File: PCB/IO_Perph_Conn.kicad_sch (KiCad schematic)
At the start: 18 parts, among them U301 STM32MP157FABx, Y601 NX2012SA-32.768K

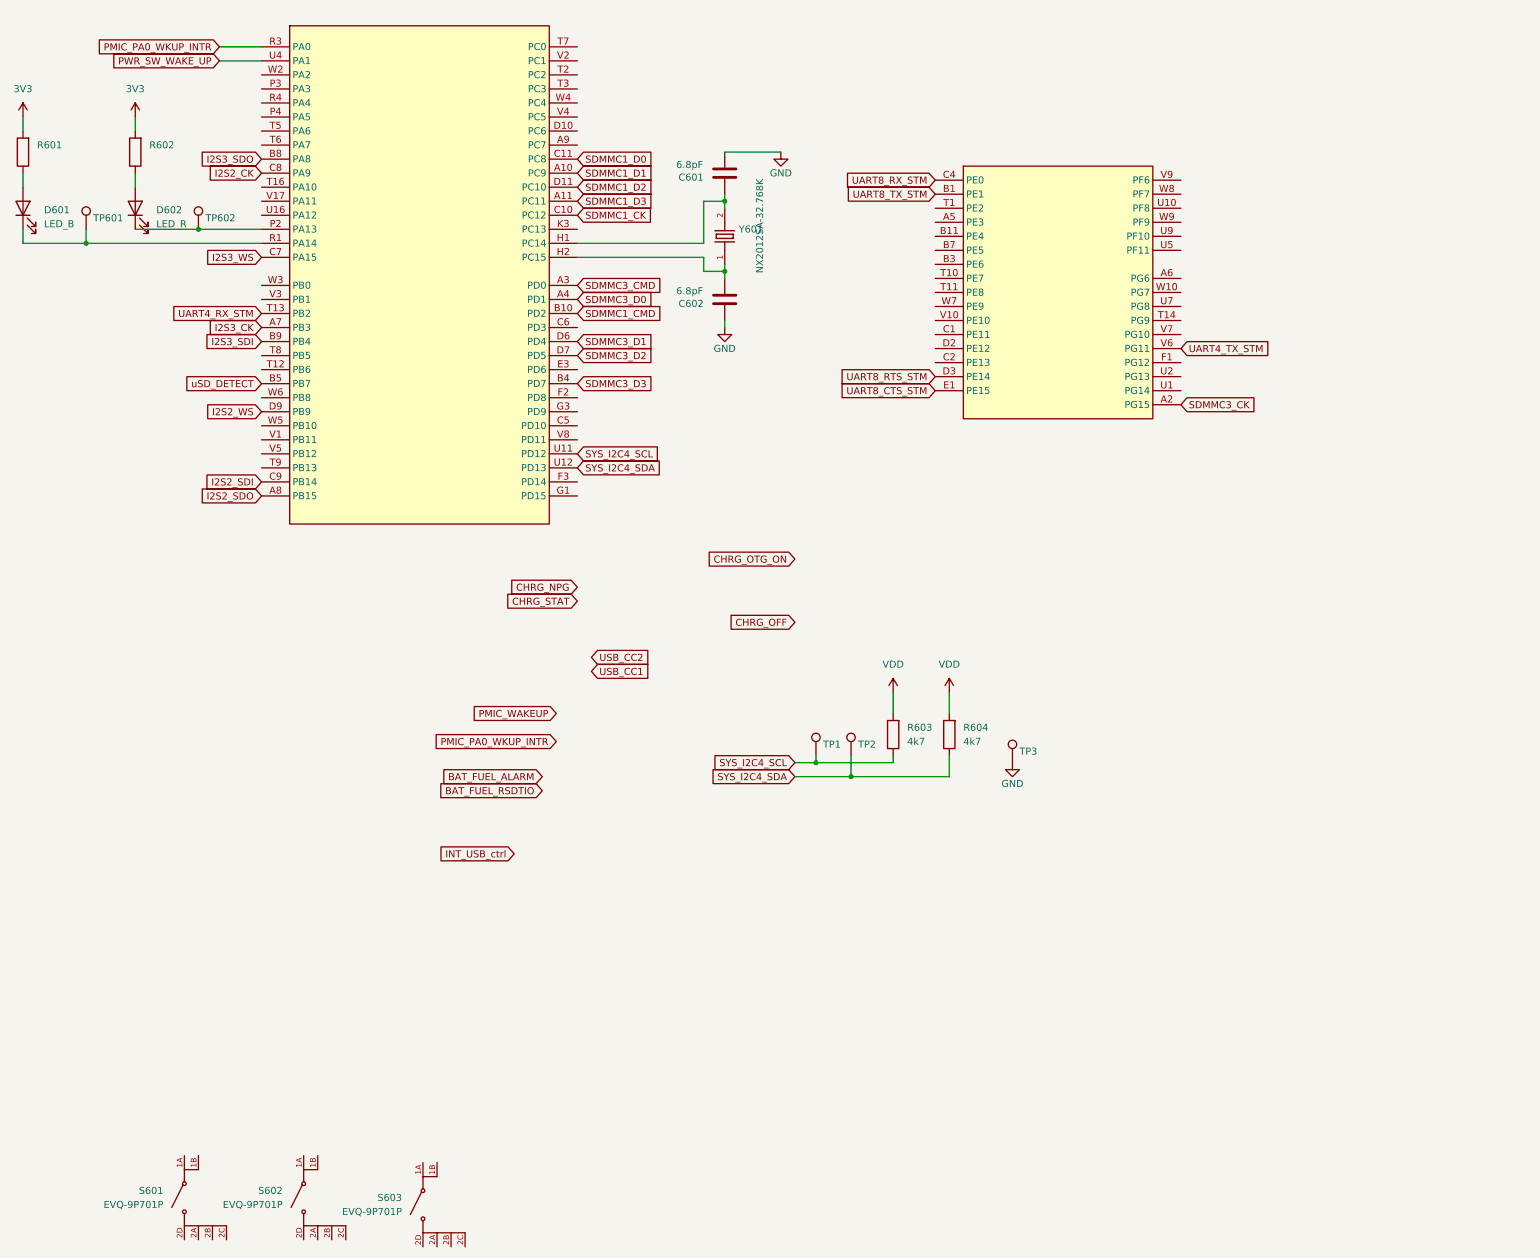
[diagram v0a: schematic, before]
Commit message: PCB_UPDATE
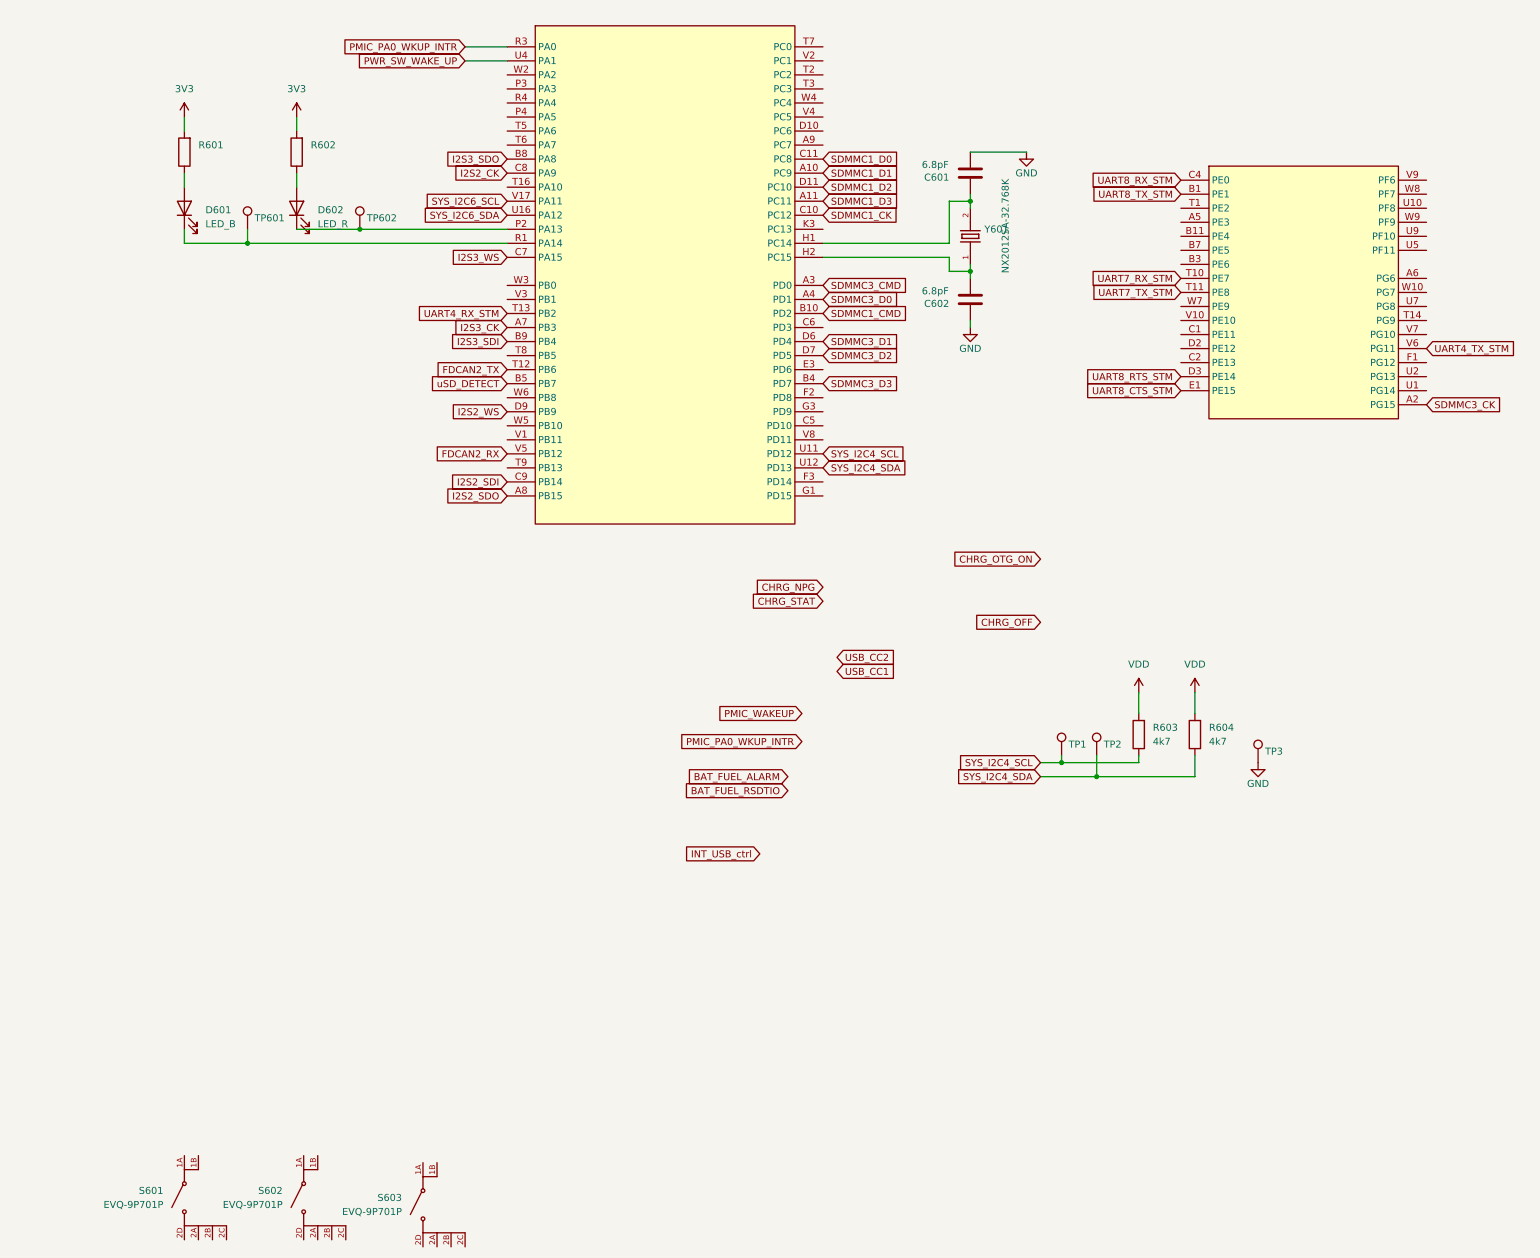
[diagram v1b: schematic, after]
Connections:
- net UART7_RX_STM: now reaches U301.T10 (PE7)
- net UART7_TX_STM: now reaches U301.T11 (PE8)
- net FDCAN2_TX: now reaches U301.T12 (PB6)
- net SYS_I2C6_SDA: now reaches U301.U16 (PA12)
- net SYS_I2C6_SCL: now reaches U301.V17 (PA11)
- net FDCAN2_RX: now reaches U301.V5 (PB12)
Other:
- moved on the sheet: C601, C602, D601, D602, R601, R602, R603, R604, TP1, TP2, TP3, TP601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

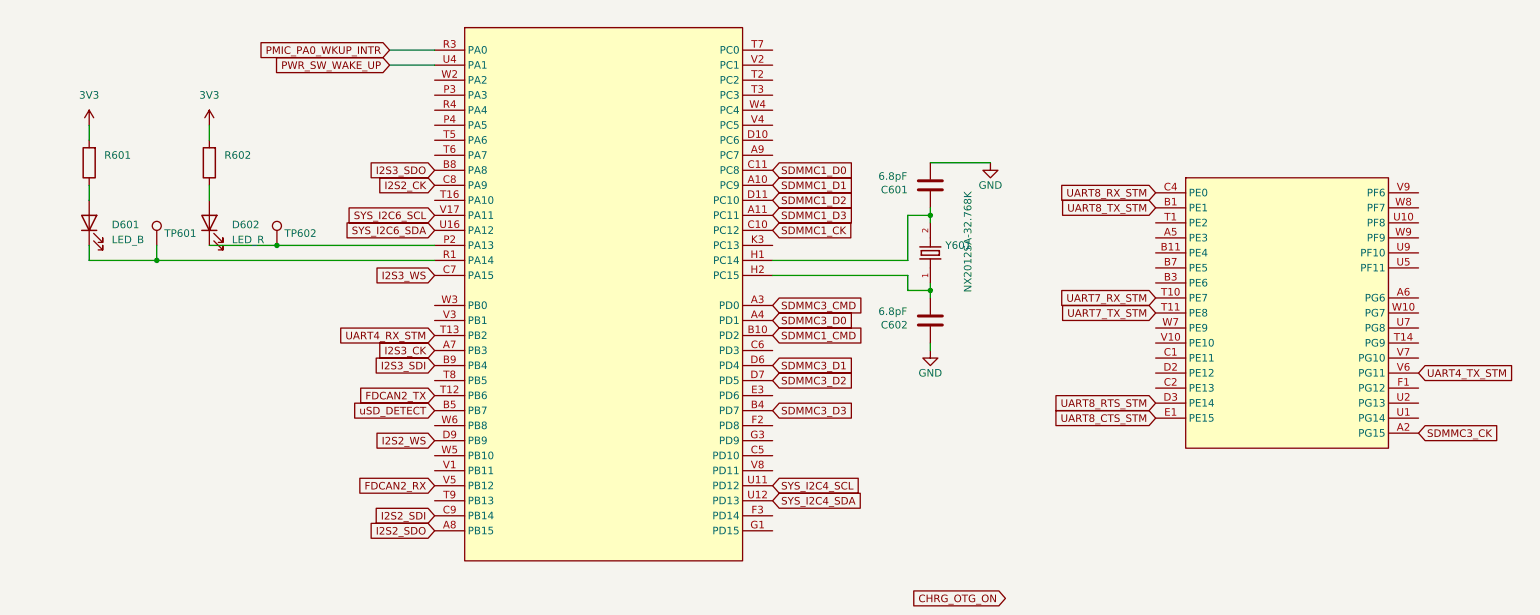
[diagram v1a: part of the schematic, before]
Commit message: psb_update
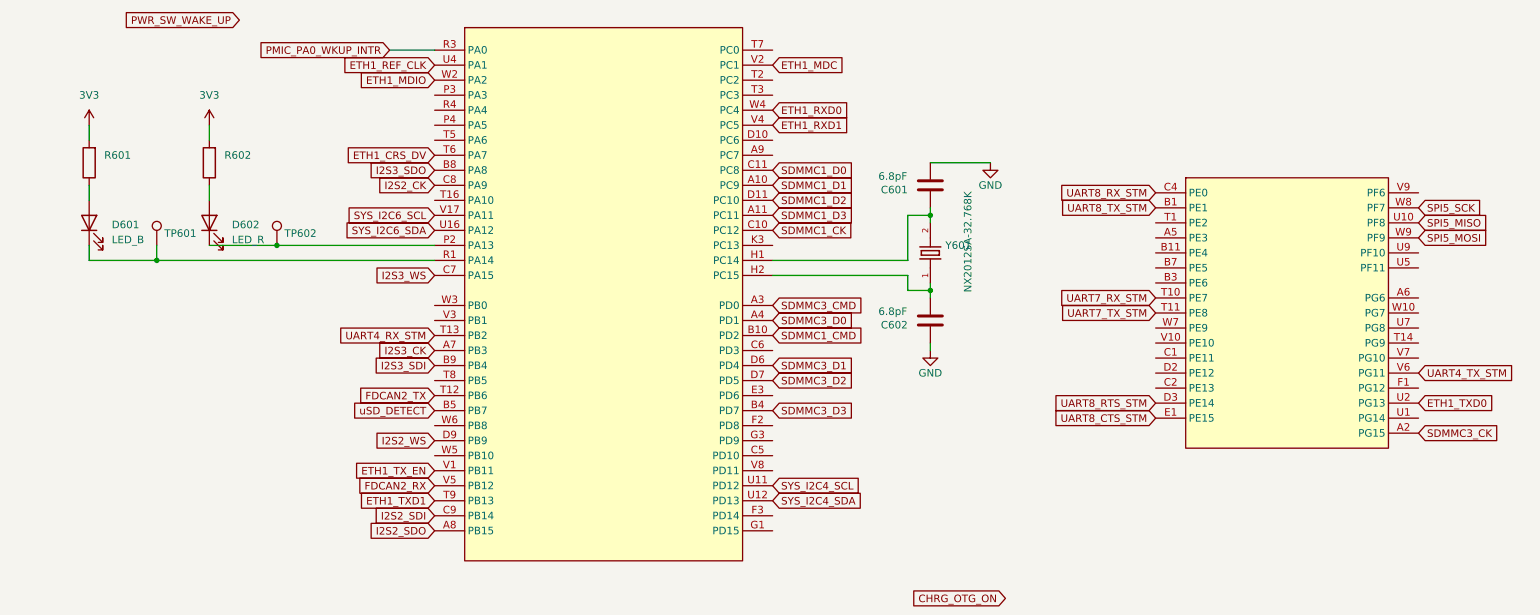
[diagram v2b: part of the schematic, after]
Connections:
- net PWR_SW_WAKE_UP: no longer U301.U4 (PA1)
- net SPI5_MISO: now reaches U301.U10 (PF8)
- net ETH1_TXD0: now reaches U301.U2 (PG13)
- net SPI5_SCK: now reaches U301.W8 (PF7)
- net SPI5_MOSI: now reaches U301.W9 (PF9)
- net ETH1_CRS_DV: now reaches U301.T6 (PA7)
- net ETH1_TXD1: now reaches U301.T9 (PB13)
- net ETH1_TX_EN: now reaches U301.V1 (PB11)
- net ETH1_MDC: now reaches U301.V2 (PC1)
- net ETH1_RXD1: now reaches U301.V4 (PC5)
- net ETH1_MDIO: now reaches U301.W2 (PA2)
- net ETH1_RXD0: now reaches U301.W4 (PC4)
- new net ETH1_REF_CLK: U301.U4 (PA1)

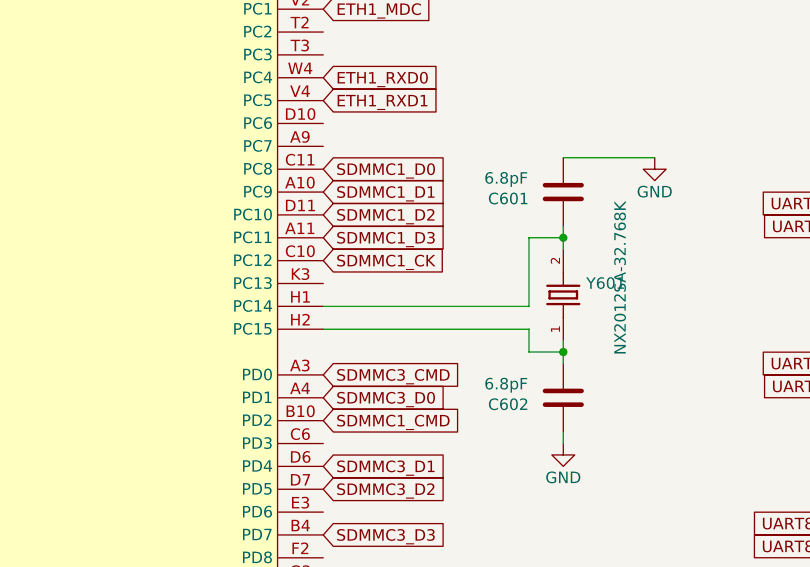
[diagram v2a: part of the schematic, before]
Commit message: PCB_UPDATE
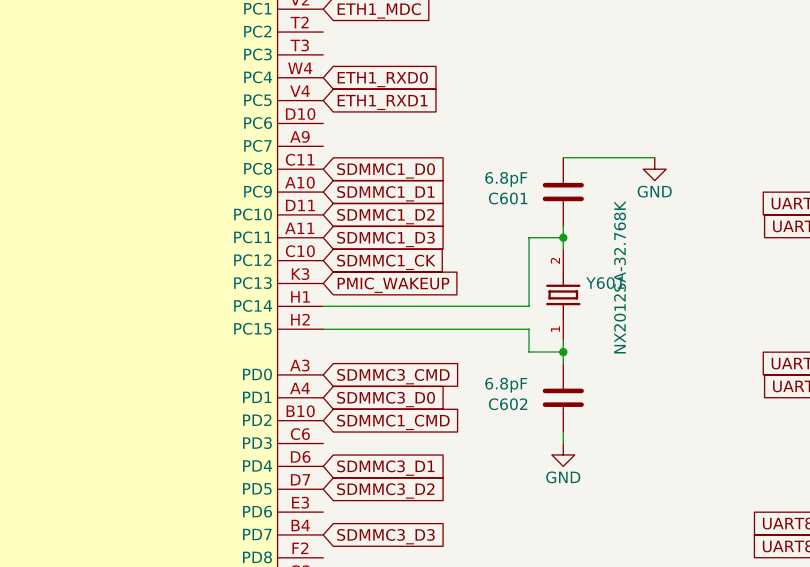
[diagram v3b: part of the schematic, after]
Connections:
- net PMIC_WAKEUP: now also U301.K3 (PC13)
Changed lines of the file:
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@@
+		)
+	)
+	(global_label "PMIC_WAKEUP"
+		(shape input)
+		(at 162.56 83.82 0)
+		(fields_autoplaced yes)
+		(effects
+			(font
+				(size 1.27 1.27)
+			)
+			(justify left)
+		)
+		(property "Intersheetrefs" "${INTERSHEET_REFS}"
+			(at 178.6685 83.82 0)
+			(effects
+				(font
+					(size 1.27 1.27)
+				)
+				(justify left)
+				(hide yes)
+			)
 		)
 	)
